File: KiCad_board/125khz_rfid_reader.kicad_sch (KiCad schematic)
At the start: 36 parts, among them J1 SPI pins, J2 UART pins, Q1 STC945, Q4 BS170, Q5 2SC9014, SW1 Switch Mode, SW2 Save Mode, U1 LM358, U2 ATmega8A-A, U4 L78L05_TO92

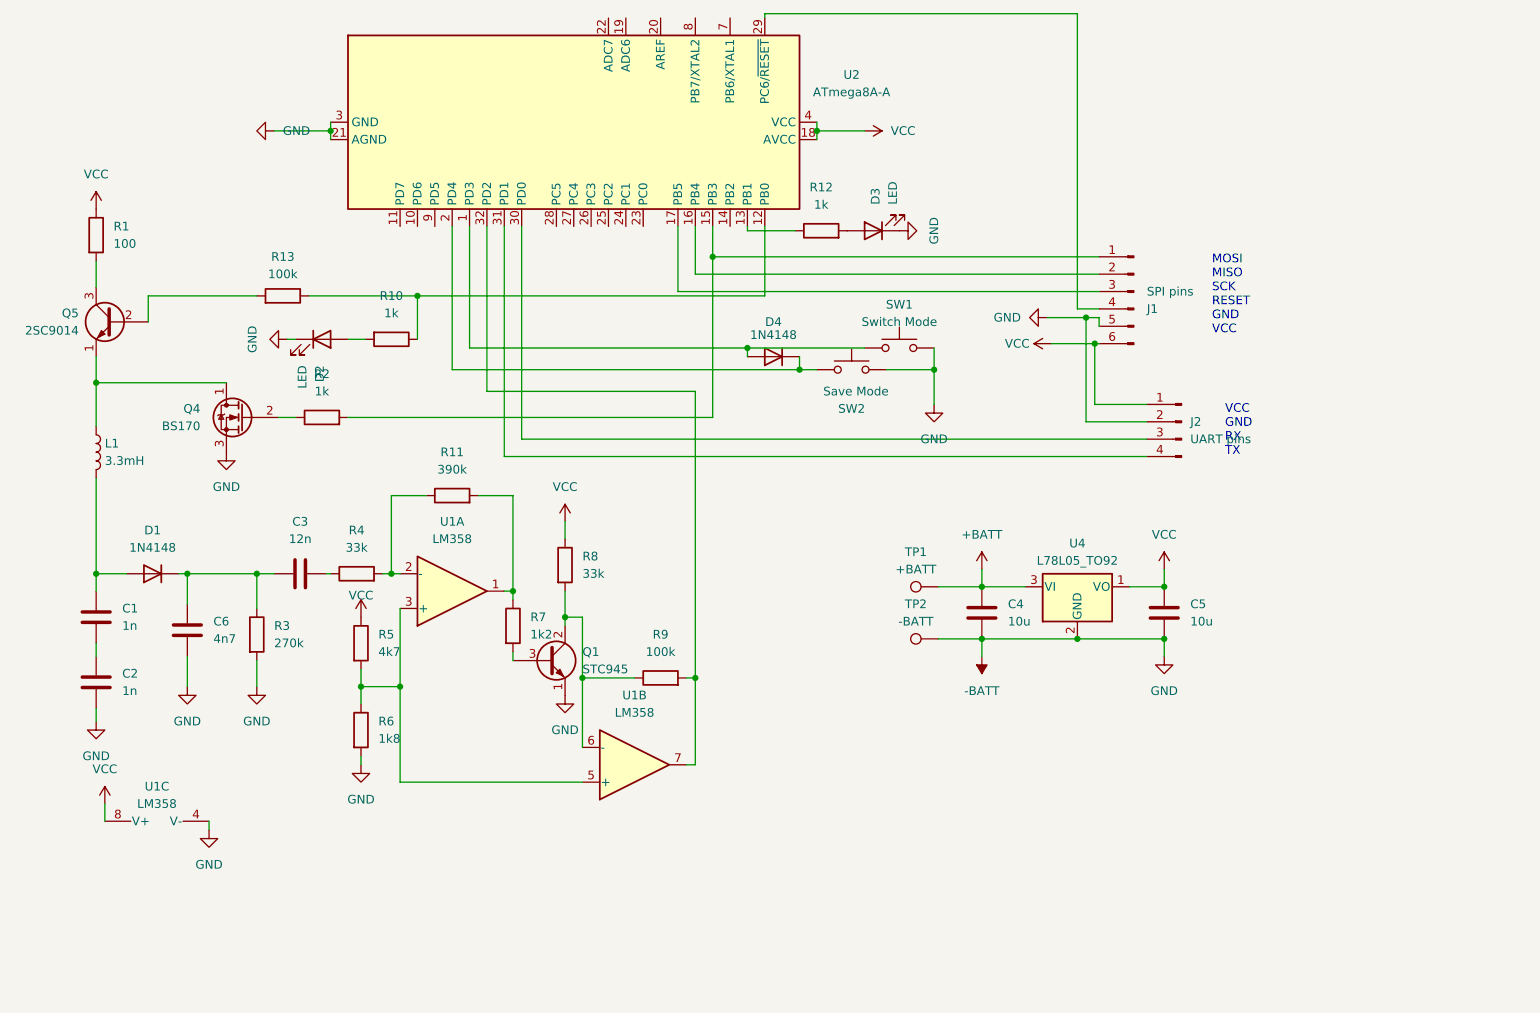
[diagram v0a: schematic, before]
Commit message: board added
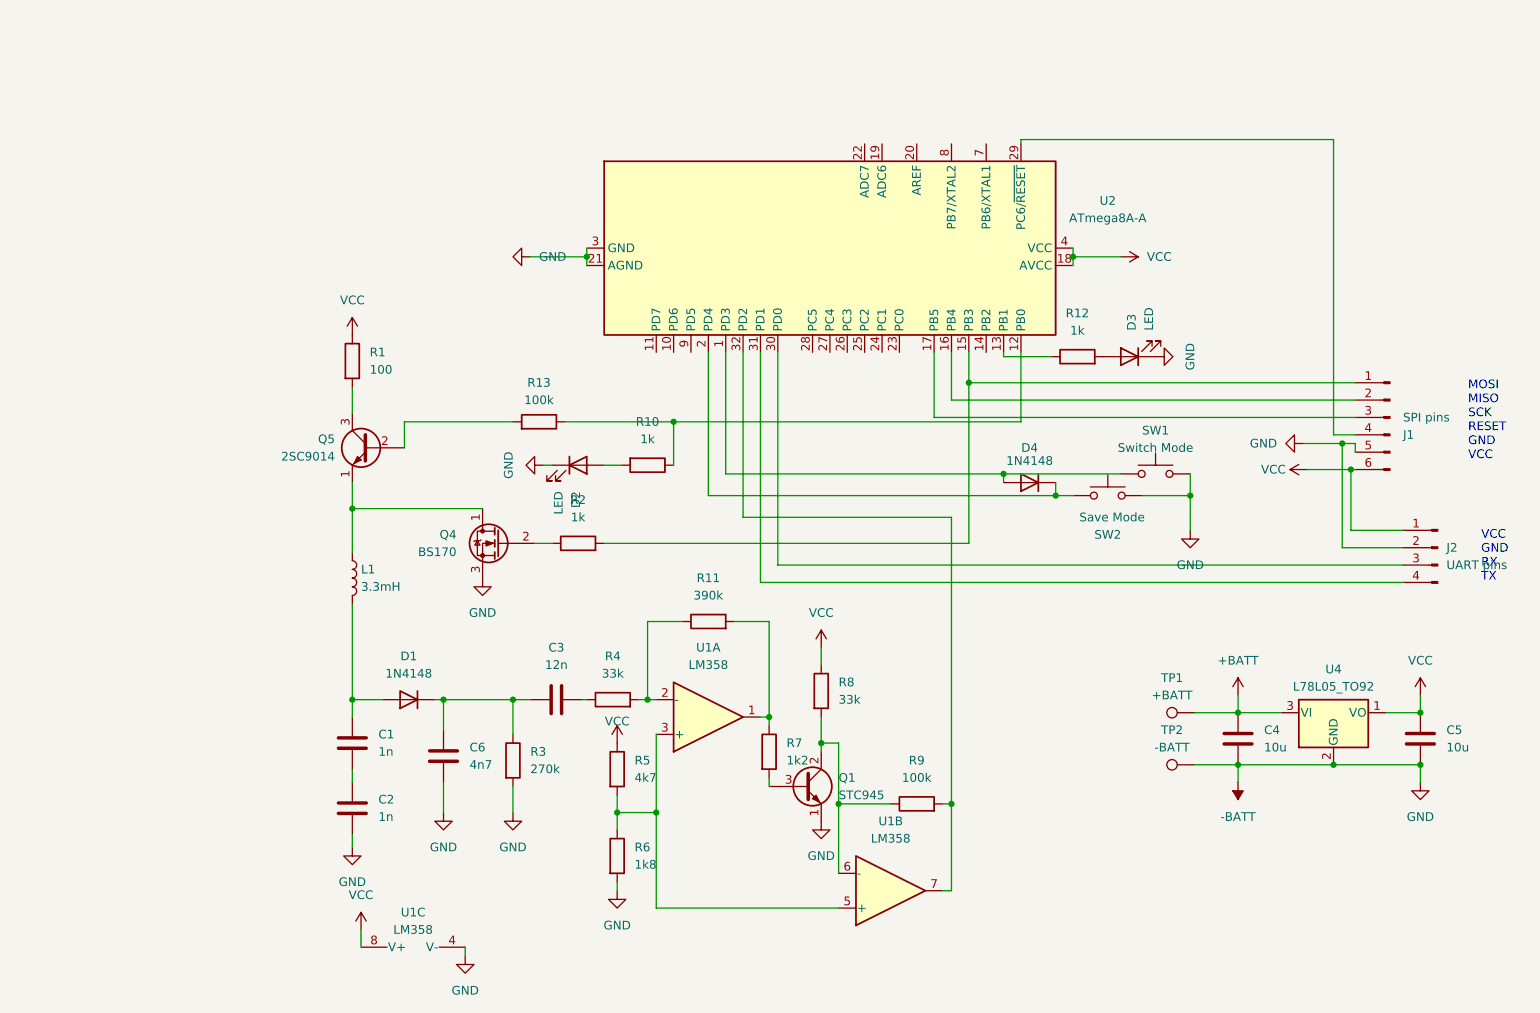
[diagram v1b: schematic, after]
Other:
- moved on the sheet: C1, C2, C3, C4, C5, C6, D1, D2, D3, D4, J1, J2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
